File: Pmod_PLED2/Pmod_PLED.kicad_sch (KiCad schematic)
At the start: 9 parts, among them IC1 TBD62064APG, J1 Barrel_Jack_Switch, J2 Conn_01x06_Pin, J3 Conn_01x03_Pin, U1 AMS1117-3.3

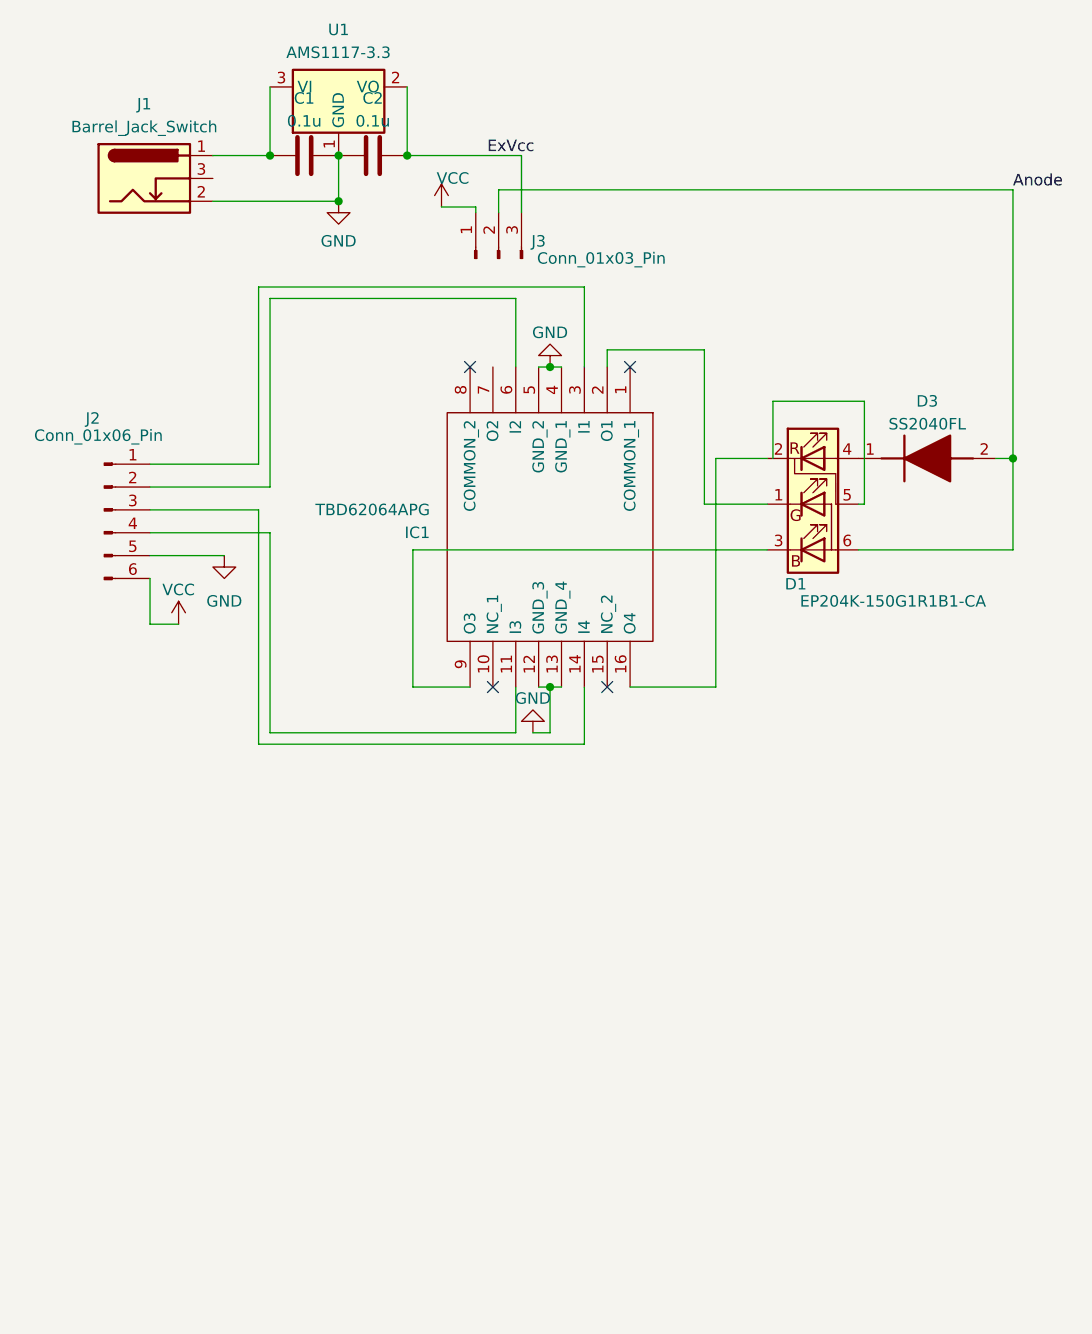
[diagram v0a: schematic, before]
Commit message: power led 2 schematics
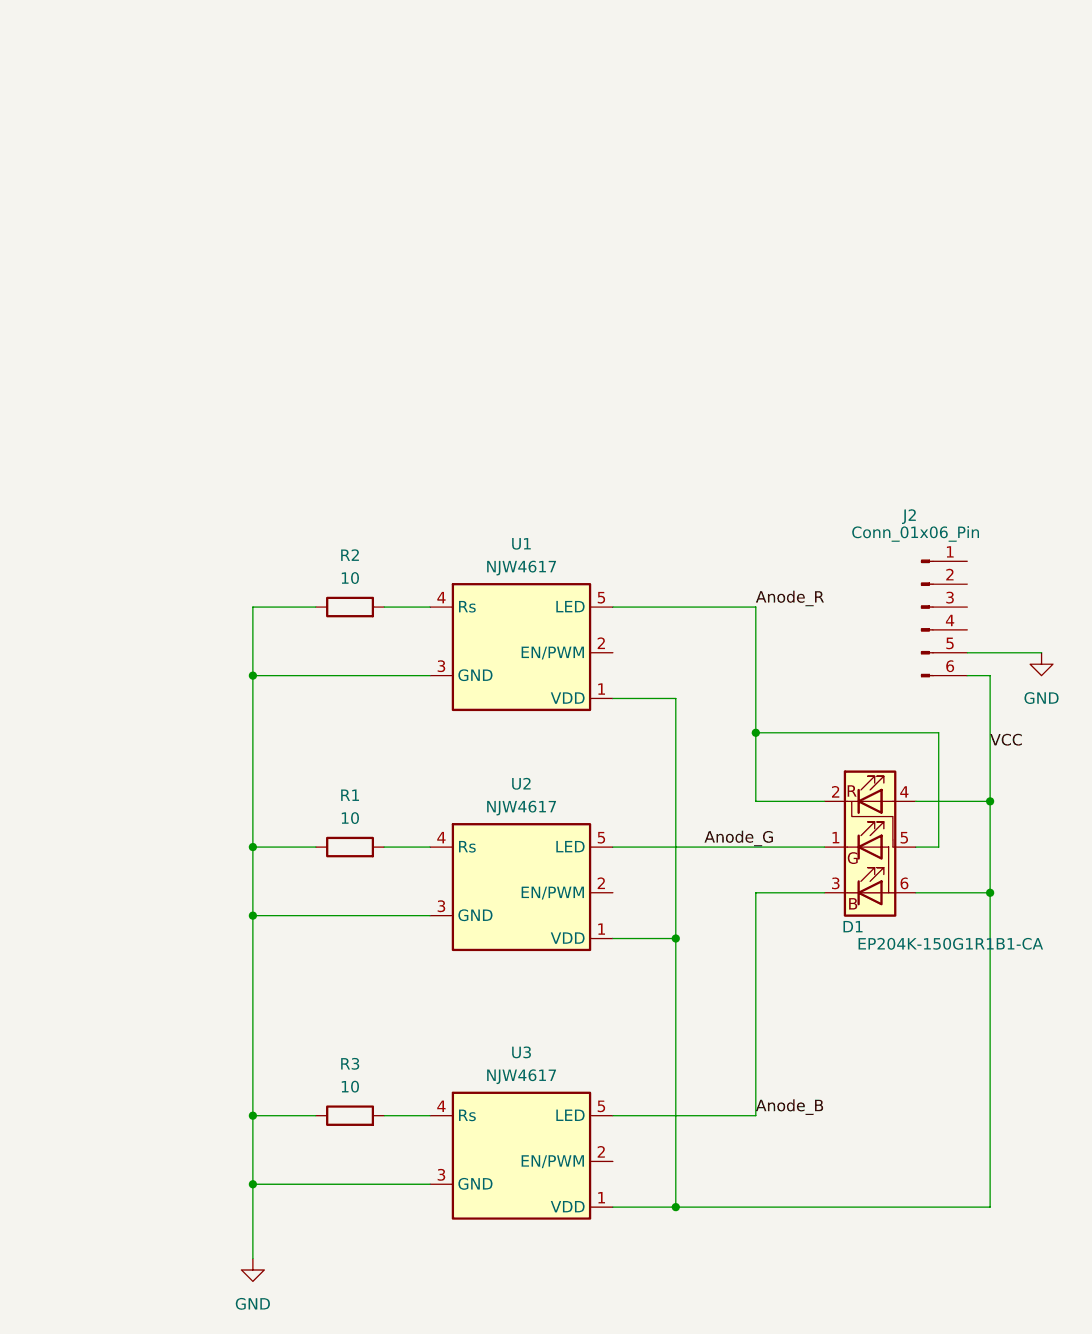
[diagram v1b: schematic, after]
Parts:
- removed C1, C2: 0.1u, Capacitor_SMD:C_0603_1608Metric_Pad1.08x0.95mm_HandSolder, symbol Device:C
- removed D3: SS2040FL, SamacSys_Parts:SODFL3618X108N, symbol SamacSys_Parts:SS2040FL
- removed IC1: TBD62064APG, SamacSys_Parts:DIP762W60P254L1975H445Q16N, symbol SamacSys_Parts:TBD62064APG
- removed J1: Barrel_Jack_Switch, Connector_BarrelJack:BarrelJack_Horizontal, symbol Connector:Barrel_Jack_Switch
- removed J3: Conn_01x03_Pin, Connector_PinHeader_2.54mm:PinHeader_1x03_P2.54mm_Vertical, symbol Connector:Conn_01x03_Pin
- removed U1: AMS1117-3.3, Package_TO_SOT_SMD:SOT-223-3_TabPin2, symbol Regulator_Linear:AMS1117-3.3
- added R1, R2, R3: 10, symbol Device:R
- added U1, U2, U3: NJW4617, Package_TO_SOT_SMD:TO-252-5_TabPin3, symbol MyLibrary:NJW4617DL3
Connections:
- net Anode is gone; now on net VCC: D1.6 (A)
- net GND: now also R1.1, R2.1, R3.1, U1.3 (GND), U2.3 (GND), U3.3 (GND)
- net VCC: now also D1.4 (RA), U1.1 (VDD), U2.1 (VDD), U3.1 (VDD)
- net Anode_G: now reaches D1.1 (GK)
- net Anode_G: now also U2.5 (LED)
- net Anode_R: now reaches D1.2 (RK)
- net Anode_R: now also D1.5 (RK), U1.5 (LED)
- net Anode_B: now reaches D1.3 (BK)
- net Anode_B: now also U3.5 (LED)
- new net: R3.2, U3.4 (Rs)
- new net: R1.2, U2.4 (Rs)
- new net: R2.2, U1.4 (Rs)
- no-connect marks 4 -> 0
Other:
- moved on the sheet: D1, J2
